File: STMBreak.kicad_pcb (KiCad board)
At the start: 2 copper layers, 31.2 x 24.6 mm, 32 parts, among them J1 Conn_01x04_Pin, J2 USB_C_Receptacle_USB2.0_14P, J3 Conn_01x06_Pin, SW1 SW_Push, U1 AMS1117-3.3, U2 AS5600, U3 STM32F103C8Tx, Y1 8M

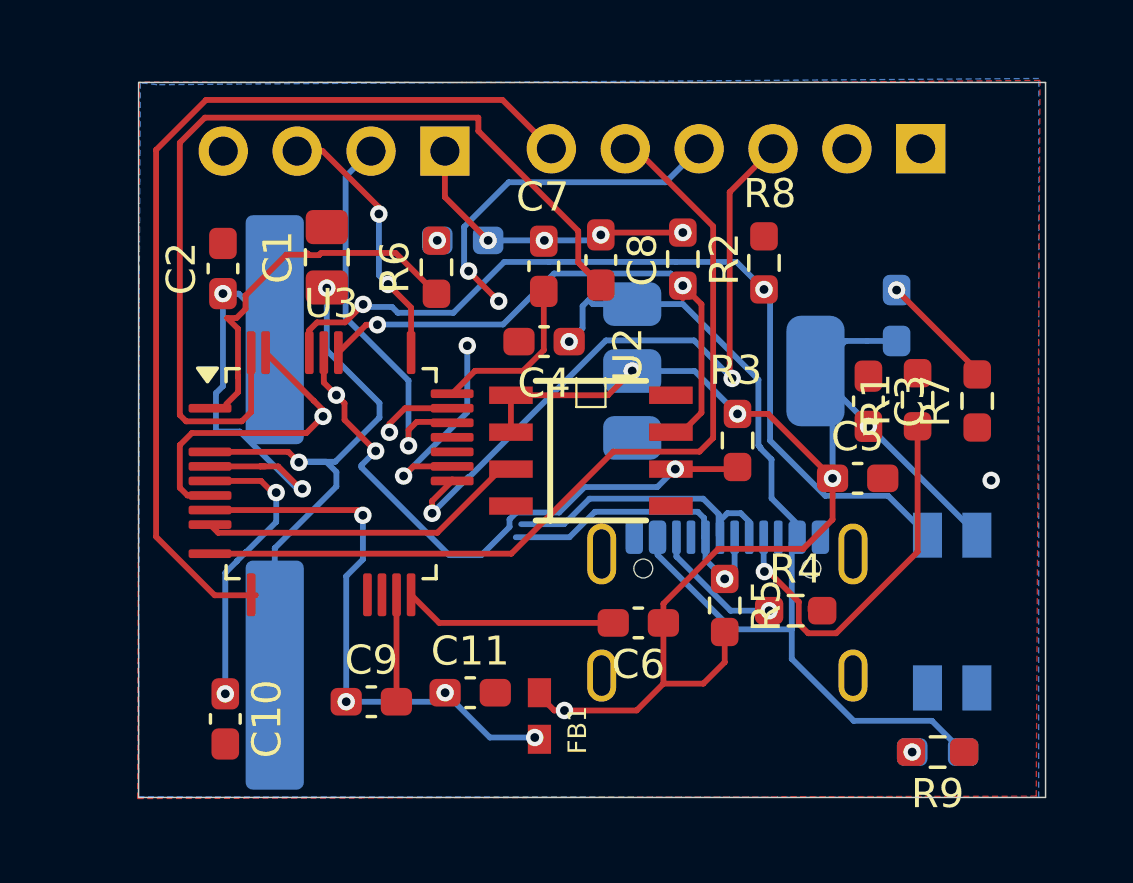
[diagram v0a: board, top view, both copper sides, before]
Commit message: Add files via upload
Modified design approach.
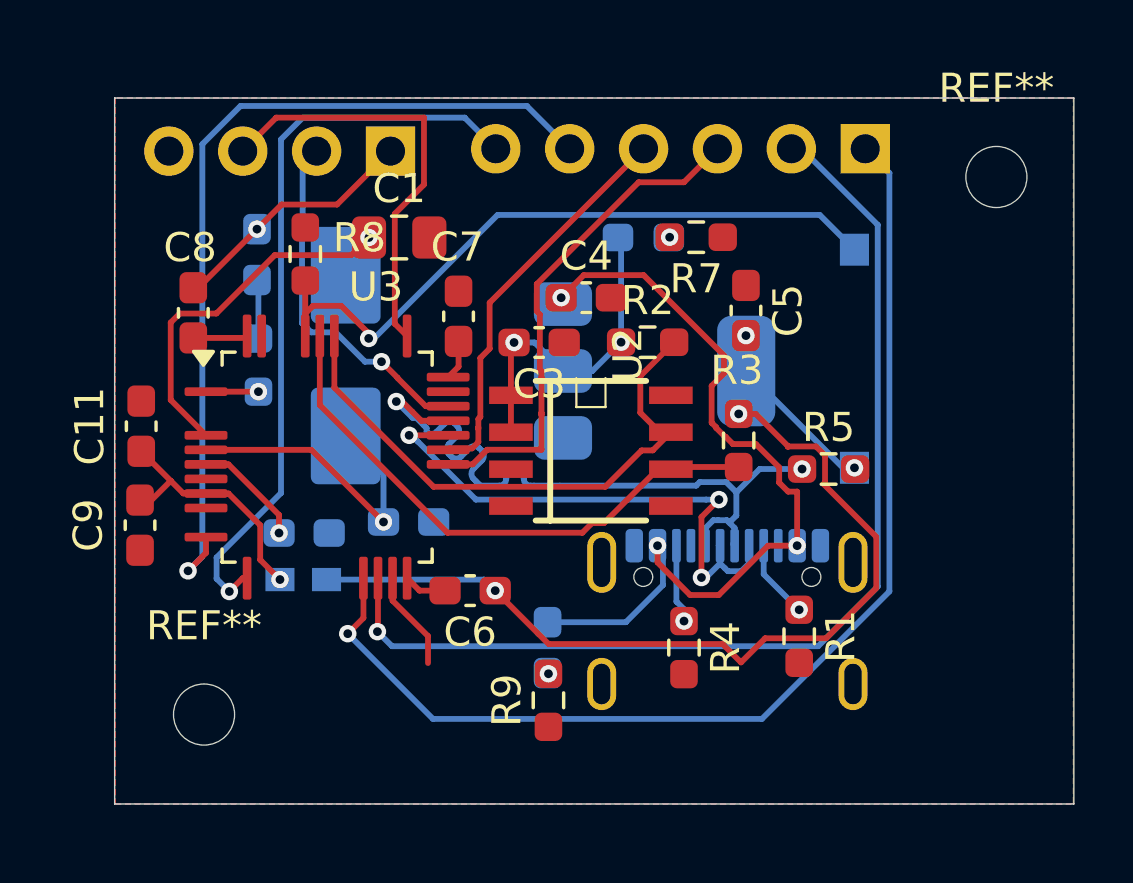
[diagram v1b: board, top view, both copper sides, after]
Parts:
- added REF**: MountingHole_2.1mm, MountingHole:MountingHole_2.1mm, F.Cu at (189.0, 72.4)
- added REF**: MountingHole_2.1mm, MountingHole:MountingHole_2.1mm, F.Cu at (161.7, 90.9)
- C10, C2, FB1, R6: moved to B.Cu
- SW1: footprint Button_Switch_SMD:Panasonic_EVQPUJ_EVQPUA -> TS09:SW_TS09-63-25-R-260-SMT-TR
- Y1: footprint Crystal:Crystal_SMD_HC49-SD_HandSoldering -> Crystal:Crystal_SMD_Abracon_ABM3-2Pin_5.0x3.2mm_HandSoldering
- moved R8 15.8 mm to (165.2, 75.1)
- moved C11 14.6 mm to (159.6, 81.0), turned to 90 degrees
- moved C8 14.1 mm to (161.4, 77.1)
- moved D3 13.9 mm to (173.6, 88.6), turned to 90 degrees
- moved R9 13.5 mm to (173.6, 90.4), turned to 90 degrees
- moved C3 11.5 mm to (173.3, 78.1), turned to 180 degrees
- moved R7 11.2 mm to (178.7, 74.5), turned to 180 degrees
- moved C2 10.8 mm to (168.8, 84.3), turned to 0 degrees
- moved C9 10.0 mm to (159.5, 84.4), turned to -90 degrees
- moved FB1 9.38 mm to (165.2, 86.2), turned to 180 degrees
- moved SW1 9.32 mm to (184.1, 78.7)
- moved D2 9.11 mm to (176.8, 74.5), turned to 180 degrees
- moved R1 9.09 mm to (182.2, 88.2), turned to -90 degrees
- moved D1 7.09 mm to (163.6, 75.1), turned to 90 degrees
- moved R6 6.98 mm to (163.6, 78.9)
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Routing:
- net I2CSCL: track 0.00 -> 39.3 mm, vias 0 -> 1
- net I2CSDA: track 0.00 -> 36.6 mm, vias 0 -> 1
- net Net-(C8-Pad2): track 33.2 -> 1.88 mm
- net GND: track 18.1 -> 3.42 mm, vias 3 -> 0
- net D+: track 10.9 -> 25.0 mm, vias 1 -> 2
- net OUT: track 11.4 -> 0.00 mm
- net VDDA: track 19.4 -> 8.62 mm, vias 4 -> 1
- net Net-(J2-CC1): track 13.3 -> 2.71 mm
- net CLED: track 12.3 -> 1.80 mm, vias 0 -> 1
- net OSCIN: track 21.2 -> 12.4 mm, vias 2 -> 1
- net D-: track 10.6 -> 19.3 mm, vias 0 -> 3
- net U2RX: track 32.6 -> 25.6 mm, vias 0 -> 1
- net Net-(U3-NRST): track 10.1 -> 3.85 mm, vias 2 -> 1
- net UTX: track 23.3 -> 17.3 mm, vias 2 -> 0
- net URX: track 19.5 -> 13.6 mm, vias 4 -> 0
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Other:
- board size 31.2 x 24.6 mm -> 33 x 24.3 mm
